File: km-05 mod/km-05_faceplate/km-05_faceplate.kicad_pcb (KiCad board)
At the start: 4 copper layers, 50.8 x 76.2 mm, 8 parts

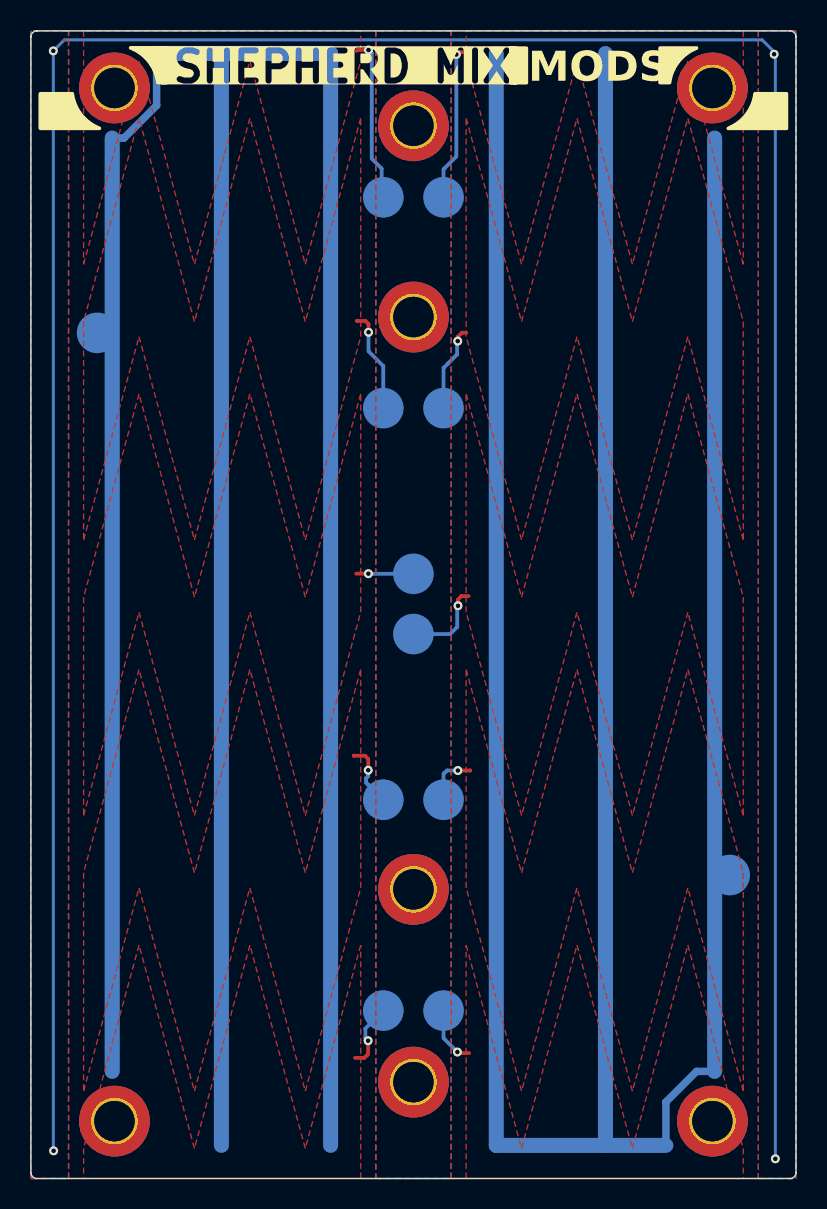
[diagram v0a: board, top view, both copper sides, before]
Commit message: n
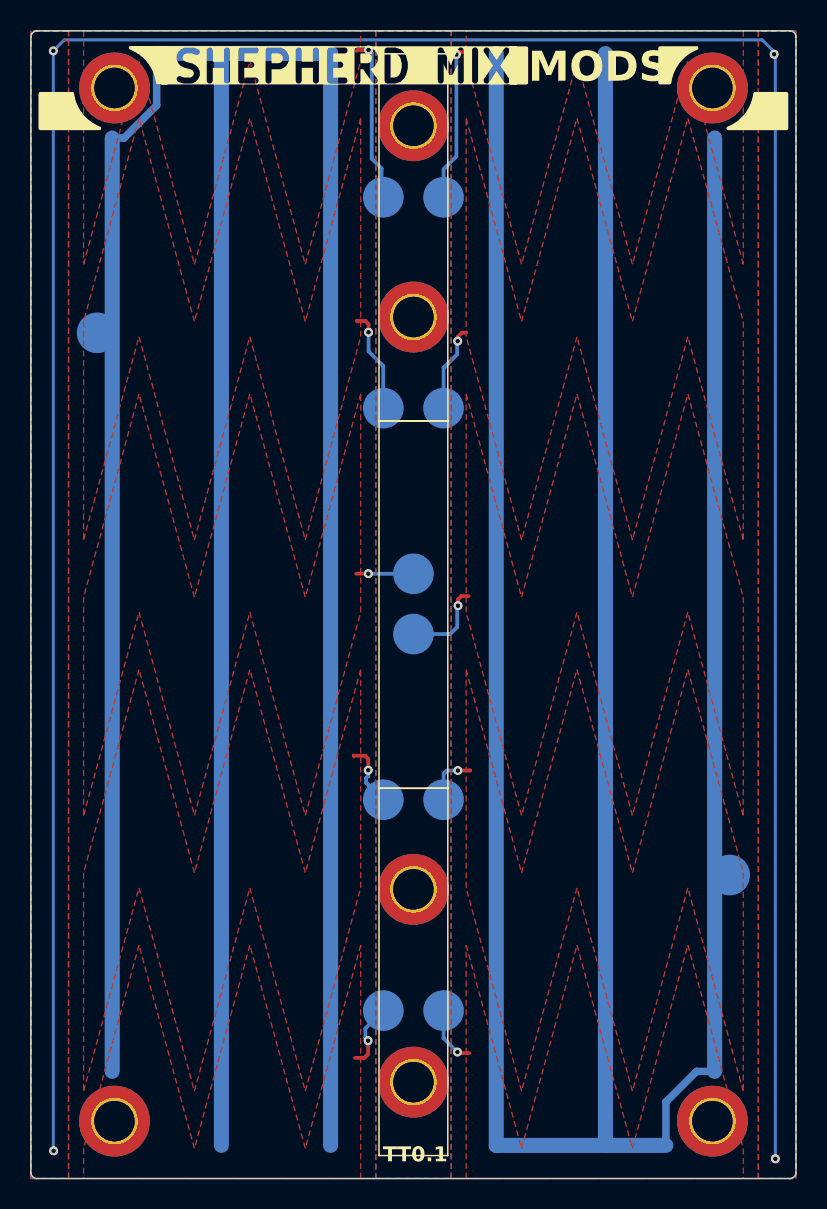
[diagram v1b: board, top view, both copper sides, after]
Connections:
- H1 pad 1: (no net) -> GND (x2)
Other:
- board text added: "TT0.1"
